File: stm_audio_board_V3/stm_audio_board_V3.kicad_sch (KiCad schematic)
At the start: 0 parts

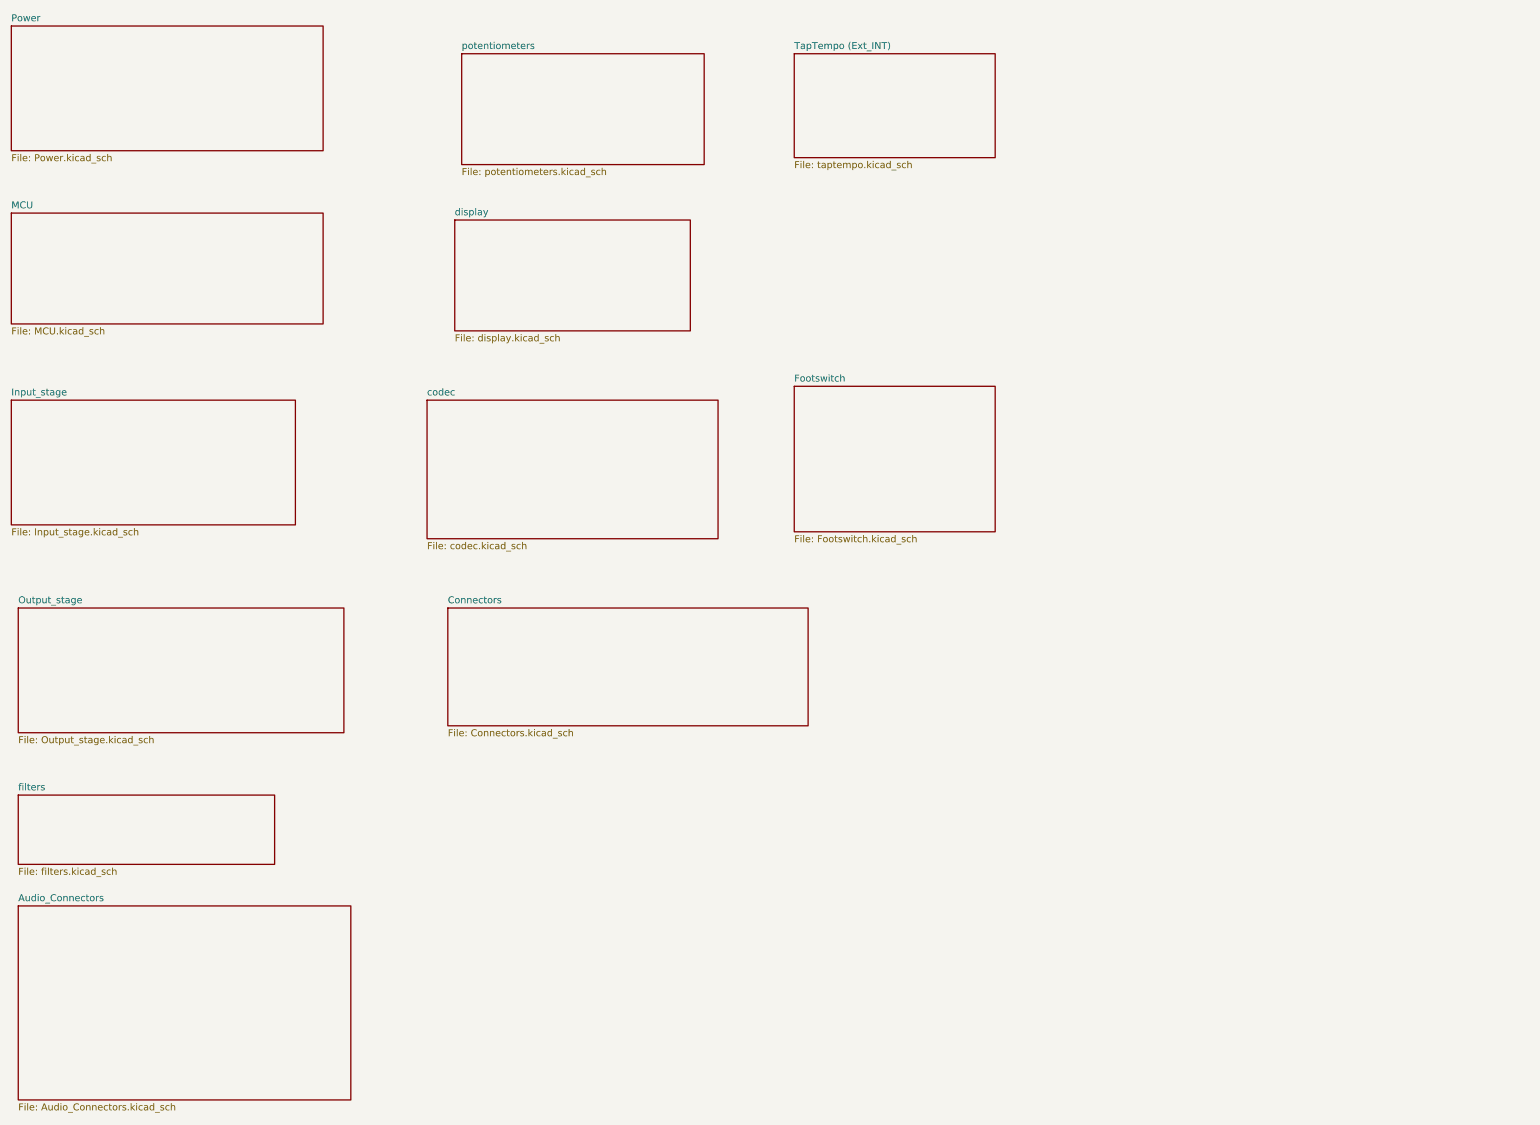
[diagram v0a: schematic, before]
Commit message: minor changes
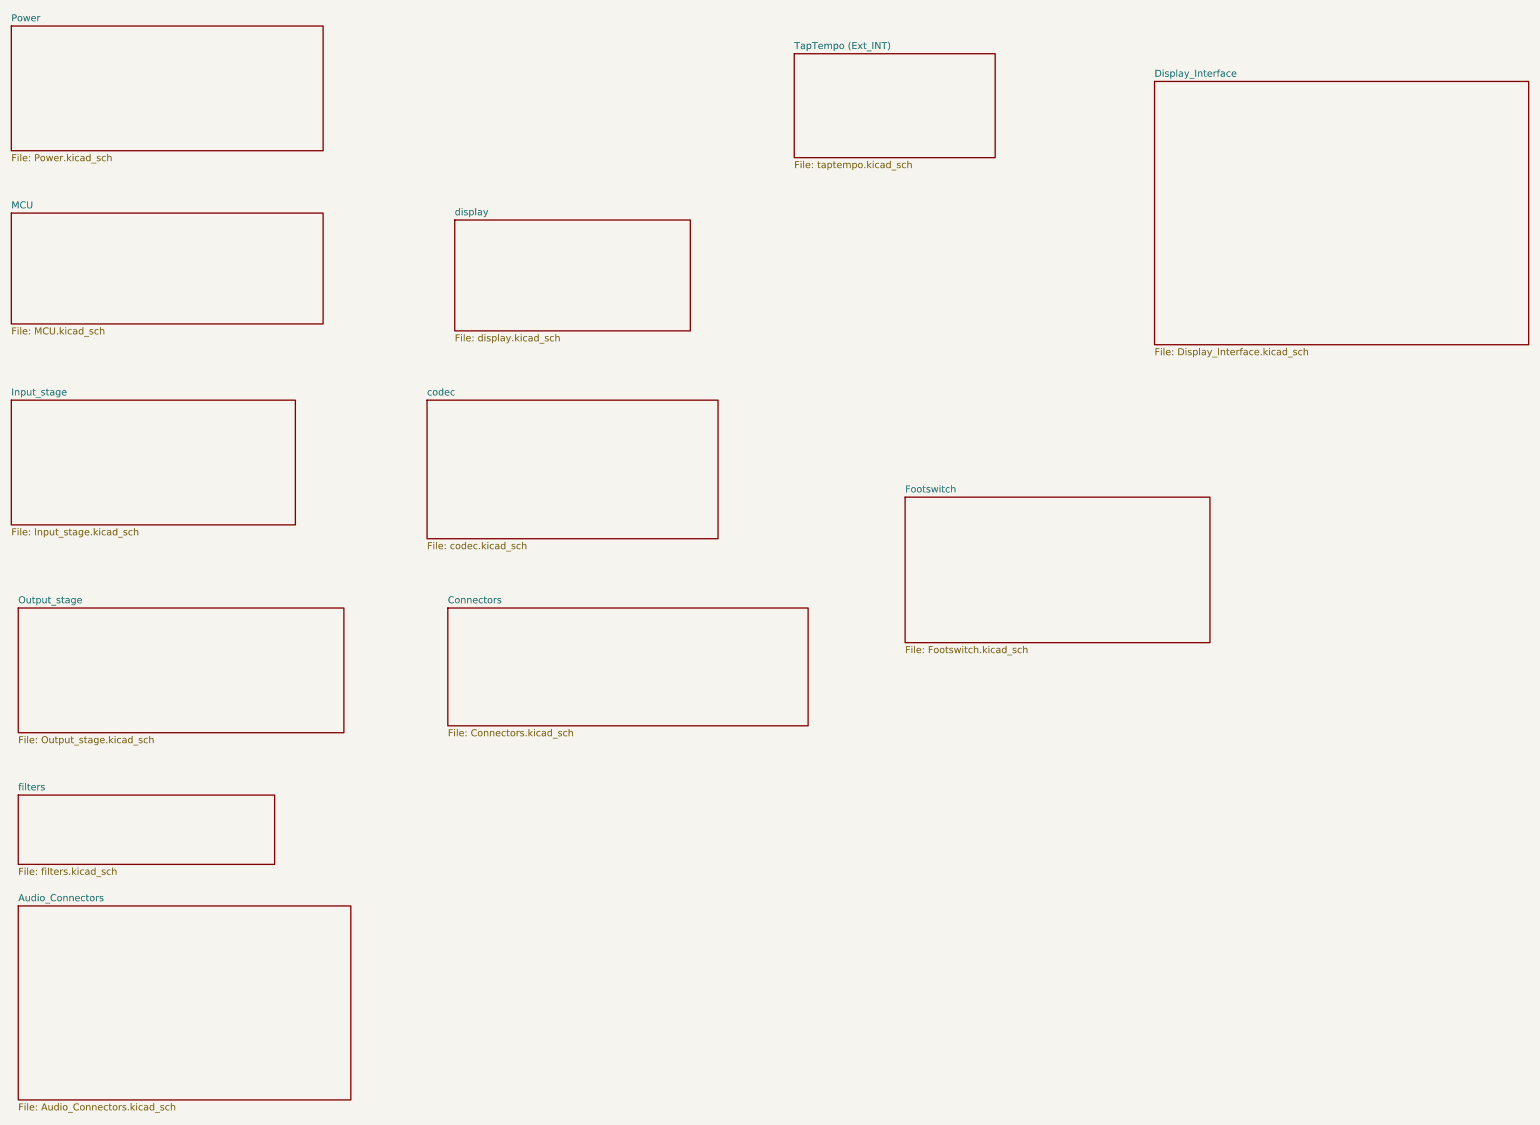
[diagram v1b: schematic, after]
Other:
- removed sheet potentiometers
- added sheet Display_Interface (Display_Interface.kicad_sch)
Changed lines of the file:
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@@
 (kicad_sch (version 20230121) (generator eeschema)
   (paper "A3")
+  (sheet (at 231.14 46.99) (size 68.58 48.26) (fields_autoplaced)
+    (stroke (width 0.1524) (type solid))
+    (fill (color 0 0 0 0.0000))
+    (property "Sheetname" "Display_Interface" (at 231.14 46.2784 0)
+      (effects (font (size 1.27 1.27)) (justify left bottom))
+    )
+    (property "Sheetfile" "Display_Interface.kicad_sch" (at 231.14 95.8346 0)
+      (effects (font (size 1.27 1.27)) (justify left top))
+    )
+    (instances
+      (project "stm_audio_board_V3"
+        (path "/6997cf63-2615-4e49-9471-e7da1b6bae71" (page "14"))
+      )
+    )
+  )
   (sheet (at 21.59 36.83) (size 57.15 22.86) (fields_autoplaced)
     (stroke (width 0.1524) (type solid))
@@
       (project "stm_audio_board_V3"
         (path "/6997cf63-2615-4e49-9471-e7da1b6bae71" (page "3"))
+      )
+    )
+  )
+  (sheet (at 185.42 123.19) (size 55.88 26.67) (fields_autoplaced)
+    (stroke (width 0.1524) (type solid))
+    (fill (color 0 0 0 0.0000))
+    (property "Sheetname" "Footswitch" (at 185.42 122.4784 0)
+      (effects (font (size 1.27 1.27)) (justify left bottom))
+    )
+    (property "Sheetfile" "Footswitch.kicad_sch" (at 185.42 150.4446 0)
+      (effects (font (size 1.27 1.27)) (justify left top))
+    )
+    (instances
+      (project "stm_audio_board_V3"
+        (path "/6997cf63-2615-4e49-9471-e7da1b6bae71" (page "12"))
+        (path "/6997cf63-2615-4e49-9471-e7da1b6bae71/027e1bfd-1867-4598-8450-c55193b376a5" (page "12"))
       )
     )
@@
     )
   )
-  (sheet (at 165.1 102.87) (size 36.83 26.67) (fields_autoplaced)
-    (stroke (width 0.1524) (type solid))
-    (fill (color 0 0 0 0.0000))
-    (property "Sheetname" "Footswitch" (at 165.1 102.1584 0)
-      (effects (font (size 1.27 1.27)) (justify left bottom))
-    )
-    (property "Sheetfile" "Footswitch.kicad_sch" (at 165.1 130.1246 0)
-      (effects (font (size 1.27 1.27)) (justify left top))
-    )
-    (instances
-      (project "stm_audio_board_V3"
-        (path "/6997cf63-2615-4e49-9471-e7da1b6bae71" (page "12"))
-      )
-    )
-  )
   (sheet (at 165.1 41.91) (size 36.83 19.05) (fields_autoplaced)
     (stroke (width 0.1524) (type solid))
@@
       )
     )
-  )
-  (sheet (at 104.14 41.91) (size 44.45 20.32) (fields_autoplaced)
-    (stroke (width 0.1524) (type solid))
-    (fill (color 0 0 0 0.0000))
-    (property "Sheetname" "potentiometers" (at 104.14 41.1984 0)
-      (effects (font (size 1.27 1.27)) (justify left bottom))
-    )
-    (property "Sheetfile" "potentiometers.kicad_sch" (at 104.14 62.8146 0)
-      (effects (font (size 1.27 1.27)) (justify left top))
-    )
-    (instances
-      (project "stm_audio_board_V3"
-        (path "/6997cf63-2615-4e49-9471-e7da1b6bae71" (page "6"))
-      )
-    )
